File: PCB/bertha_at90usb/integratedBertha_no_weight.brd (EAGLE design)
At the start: 108.1 x 84.6 mm, 92 parts, among them CON1 SPI, IC1 REG1117, J1 RJ12, J2 RJ12, J3 RJ12, J4 RJ12, J5 RJ12, J7 22--02, Q1 BSP75, Q2 BSP75, Q4 BSP75, Q5 BSP75, Q6 BSP75, Q7 IRF3704S, X2 22-23-20315.08S, X3 16MHz, X4 MINI-USB, X5 22-23-20315.08S, X6 87758-4016

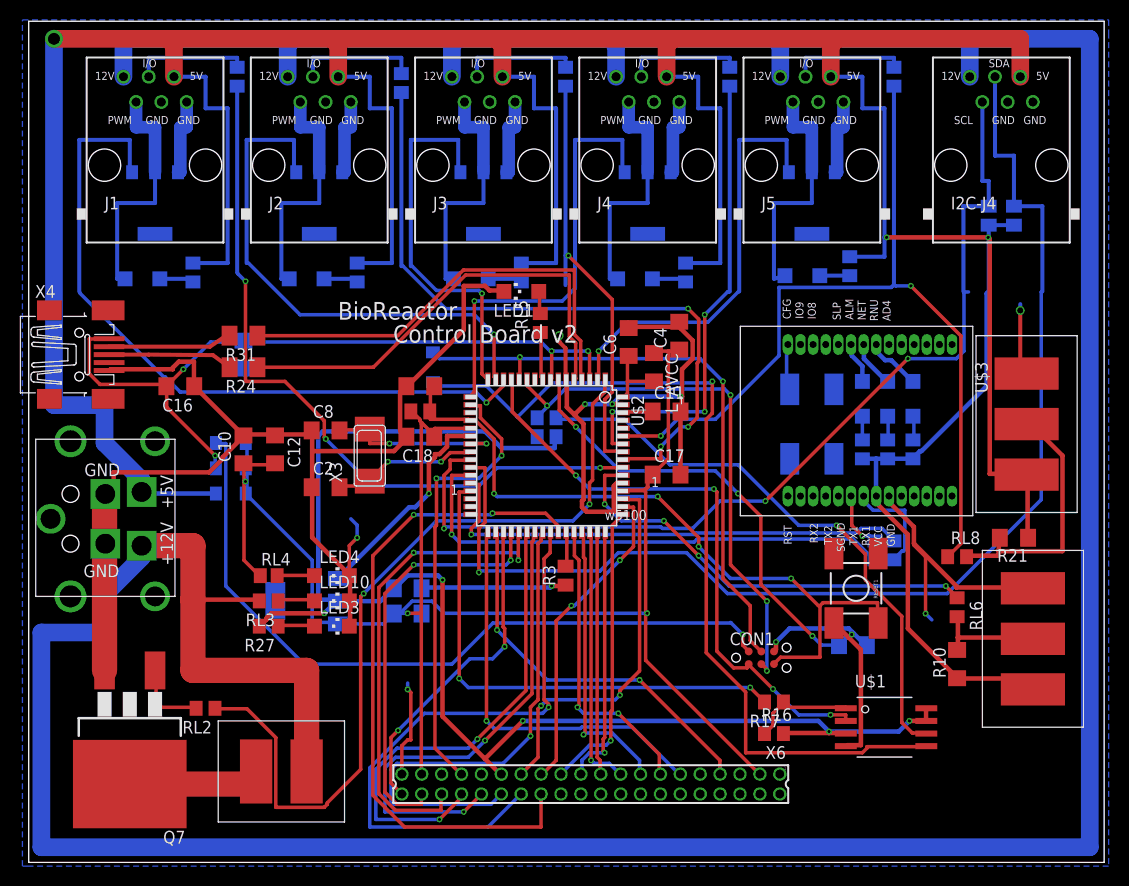
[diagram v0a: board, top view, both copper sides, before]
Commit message: Re-added mass line for security
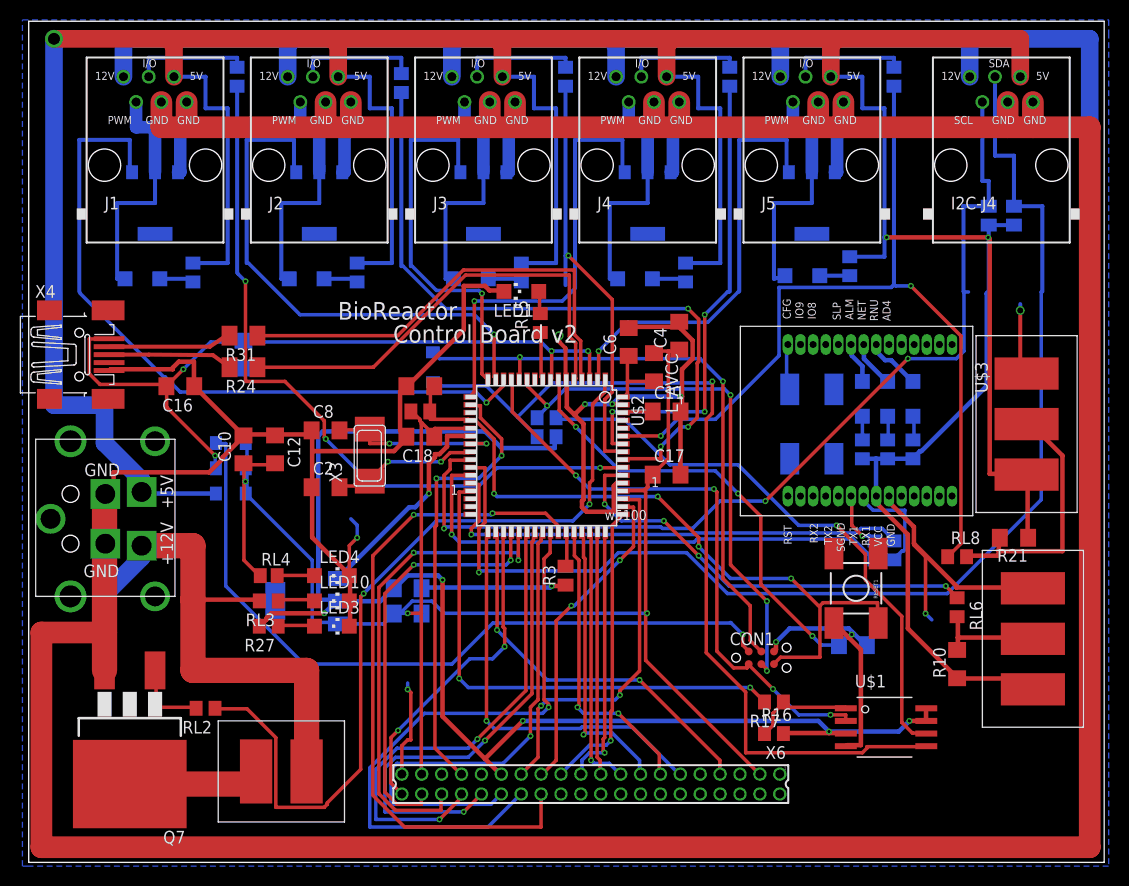
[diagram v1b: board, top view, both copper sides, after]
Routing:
- net GND: track 344.2 -> 673.8 mm
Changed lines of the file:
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@@
 <contactref element="X5" pad="3"/>
 <wire x1="7.7" y1="34.25" x2="7.62" y2="34.25" width="2.54" layer="1"/>
-<wire x1="7.62" y1="34.25" x2="7.62" y2="16.51" width="2.54" layer="1"/>
+<wire x1="7.62" y1="34.25" x2="7.62" y2="20.32" width="2.54" layer="1"/>
 <contactref element="LED1" pad="C"/>
 <contactref element="C2" pad="1"/>
@@
 <contactref element="R3" pad="1"/>
 <contactref element="X6" pad="39"/>
+<wire x1="7.62" y1="20.32" x2="7.62" y2="16.51" width="2.54" layer="1"/>
 <wire x1="16.764" y1="44.958" x2="16.64" y2="45.085" width="0.4572" layer="1"/>
 <wire x1="14.478" y1="46.7868" x2="8.2296" y2="46.7868" width="0.4572" layer="1"/>
@@
 <wire x1="39.5" y1="24.765" x2="39.5" y2="22.225" width="0" layer="19" extent="16-16"/>
 <wire x1="81.407" y1="34.036" x2="86.487" y2="34.036" width="0" layer="19" extent="1-1"/>
+<wire x1="7.62" y1="20.32" x2="1.27" y2="20.32" width="2.1844" layer="1"/>
+<wire x1="1.27" y1="20.32" x2="1.27" y2="-1.27" width="2.1844" layer="1"/>
+<wire x1="1.27" y1="-1.27" x2="106.68" y2="-1.27" width="2.1844" layer="1"/>
+<wire x1="106.68" y1="-1.27" x2="106.68" y2="71.12" width="2.1844" layer="1"/>
+<wire x1="106.68" y1="71.12" x2="100.965" y2="71.12" width="2.1844" layer="1"/>
+<wire x1="100.965" y1="71.12" x2="98.425" y2="71.12" width="2.1844" layer="1"/>
+<wire x1="98.425" y1="71.12" x2="81.915" y2="71.12" width="2.1844" layer="1"/>
+<wire x1="81.915" y1="71.12" x2="79.375" y2="71.12" width="2.1844" layer="1"/>
+<wire x1="79.375" y1="71.12" x2="65.405" y2="71.12" width="2.1844" layer="1"/>
+<wire x1="65.405" y1="71.12" x2="62.865" y2="71.12" width="2.1844" layer="1"/>
+<wire x1="62.865" y1="71.12" x2="48.895" y2="71.12" width="2.1844" layer="1"/>
+<wire x1="48.895" y1="71.12" x2="46.355" y2="71.12" width="2.1844" layer="1"/>
+<wire x1="46.355" y1="71.12" x2="32.385" y2="71.12" width="2.1844" layer="1"/>
+<wire x1="32.385" y1="71.12" x2="29.845" y2="71.12" width="2.1844" layer="1"/>
+<wire x1="29.845" y1="71.12" x2="15.875" y2="71.12" width="2.1844" layer="1"/>
+<wire x1="15.875" y1="71.12" x2="13.335" y2="71.12" width="2.1844" layer="1"/>
+<wire x1="13.335" y1="71.12" x2="13.335" y2="73.66" width="2.1844" layer="1"/>
+<wire x1="15.875" y1="71.12" x2="15.875" y2="73.66" width="2.1844" layer="1"/>
+<wire x1="29.845" y1="71.12" x2="29.845" y2="73.66" width="2.1844" layer="1"/>
+<wire x1="32.385" y1="71.12" x2="32.385" y2="73.66" width="2.1844" layer="1"/>
+<wire x1="46.355" y1="71.12" x2="46.355" y2="73.66" width="2.1844" layer="1"/>
+<wire x1="48.895" y1="71.12" x2="48.895" y2="73.66" width="2.1844" layer="1"/>
+<wire x1="62.865" y1="71.12" x2="62.865" y2="73.66" width="2.1844" layer="1"/>
+<wire x1="65.405" y1="71.12" x2="65.405" y2="73.66" width="2.1844" layer="1"/>
+<wire x1="79.375" y1="71.12" x2="79.375" y2="73.66" width="2.1844" layer="1"/>
+<wire x1="81.915" y1="71.12" x2="81.915" y2="73.66" width="2.1844" layer="1"/>
+<wire x1="98.425" y1="71.12" x2="98.425" y2="73.66" width="2.1844" layer="1"/>
+<wire x1="100.965" y1="71.12" x2="100.965" y2="73.66" width="2.1844" layer="1"/>
 </signal>
 <signal name="SCK">
